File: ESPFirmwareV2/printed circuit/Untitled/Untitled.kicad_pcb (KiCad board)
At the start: 2 copper layers, 210 x 130 mm, 2 parts

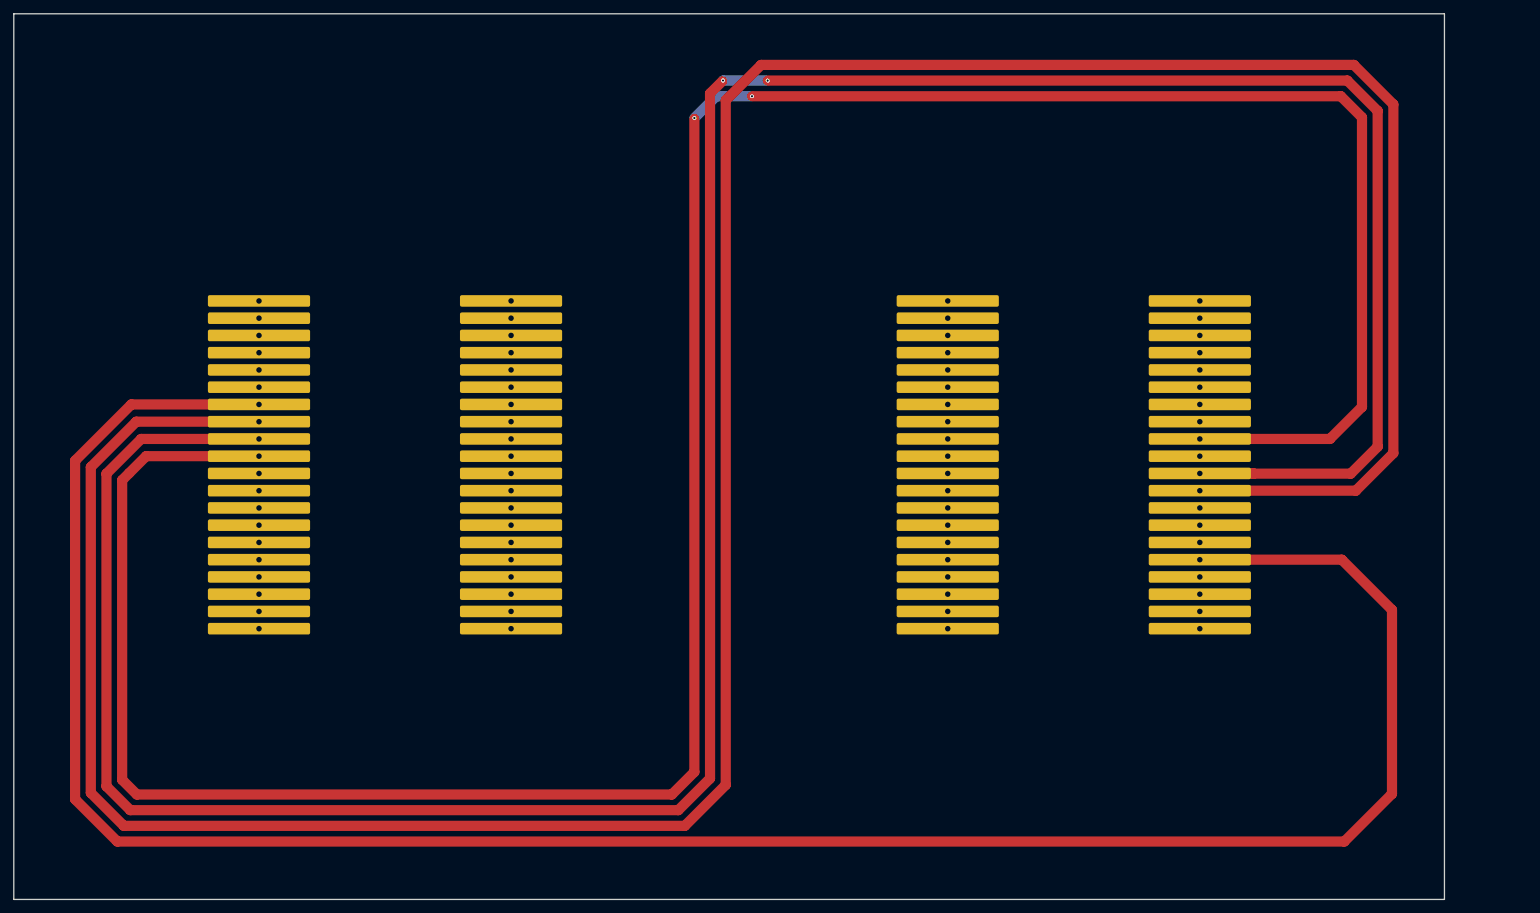
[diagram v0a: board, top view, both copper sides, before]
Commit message: backup pcb 2
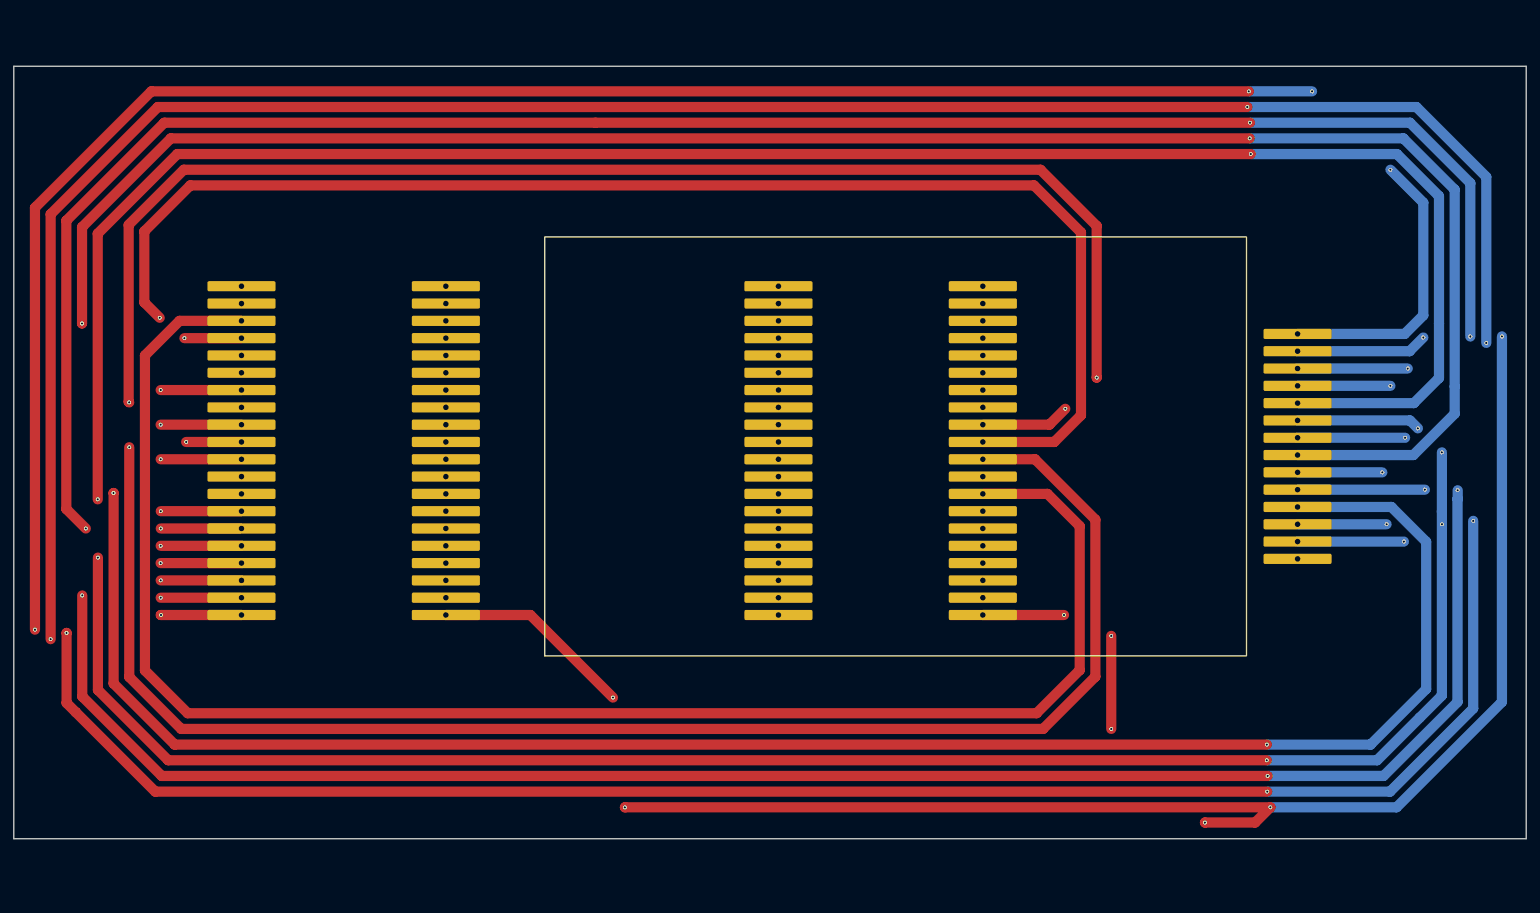
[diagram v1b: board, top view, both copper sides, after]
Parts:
- added U3: ~, customespfootprint:ili9488, F.Cu at (169.3, 92.8)
- moved U2 28.3 mm to (164.6, 93.4)
- moved U1 6.09 mm to (85.8, 93.4)
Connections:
- U1 pad 20: unconnected-(U1-GND-Pad20) -> Net-(U1-GND)
- U1 pad 23: unconnected-(U1-GPIO4-Pad23) -> Net-(U1-GPIO4)
- U1 pad 24: unconnected-(U1-GPIO5-Pad24) -> Net-(U1-GPIO5)
- U1 pad 28: Net-(U1-GPIO16) -> unconnected-(U1-GPIO16-Pad28)
- U1 pad 31: unconnected-(U1-GPIO8-Pad31) -> Net-(U1-GPIO8)
- U1 pad 34: unconnected-(U1-GPIO9-Pad34) -> Net-(U1-GPIO9)
- U1 pad 35: unconnected-(U1-GPIO10-Pad35) -> Net-(U1-GPIO10)
- U1 pad 36: unconnected-(U1-GPIO11-Pad36) -> Net-(U1-GPIO11)
- U1 pad 37: unconnected-(U1-GPIO12-Pad37) -> Net-(U1-GPIO12)
- U1 pad 38: unconnected-(U1-GPIO13-Pad38) -> Net-(U1-GPIO13)
- U1 pad 39: unconnected-(U1-GPIO14-Pad39) -> Net-(U1-GPIO14)
- U1 pad 40: unconnected-(U1-5V-Pad40) -> Net-(U1-5V)
- U2 pad 10: unconnected-(U2-GPIO5-Pad10) -> Net-(U1-GPIO5)
- U2 pad 12: Net-(U1-GPIO16) -> unconnected-(U2-GPIO16-Pad12)
- U2 pad 13: unconnected-(U2-GPIO4-Pad13) -> Net-(U1-GPIO4)
- U2 pad 16: Net-(U1-GPIO15) -> unconnected-(U2-GPIO15-Pad16)
- U2 pad 20: unconnected-(U2-GND-Pad20) -> Net-(U1-GND)
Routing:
- net Net-(U1-GPIO16): track 457.9 -> 0.00 mm
- net Net-(U1-GPIO14): track 0.00 -> 370.2 mm, vias 0 -> 5
- net Net-(U1-5V): track 0.00 -> 352.5 mm, vias 0 -> 5
- net Net-(U1-GPIO13): track 0.00 -> 339.4 mm, vias 0 -> 6
- net Net-(U1-GPIO10): track 0.00 -> 334.8 mm, vias 0 -> 5
- net Net-(U1-GPIO12): track 0.00 -> 332.7 mm, vias 0 -> 6
- net Net-(U1-GND): track 0.00 -> 331.8 mm, vias 0 -> 9
- net Net-(U1-GPIO11): track 0.00 -> 326.7 mm, vias 0 -> 7
- net Net-(U1-GPIO9): track 0.00 -> 314.1 mm, vias 0 -> 3
- net Net-(U1-GPIO8): track 0.00 -> 291.9 mm, vias 0 -> 3
- net Net-(U1-GPIO4): track 0.00 -> 242.3 mm
- net Net-(U1-GPIO5): track 0.00 -> 212.9 mm, vias 0 -> 2
- net Net-(U1-GPIO17): track 440.5 -> 243.0 mm
- net Net-(U1-GPIO18): track 416.5 -> 236.9 mm, vias 2 -> 4
- net Net-(U1-GPIO15): track 337.1 -> 313.0 mm, vias 0 -> 3
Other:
- board size 210 x 130 mm -> 222 x 113.4 mm
- copper layers 2 -> 4
